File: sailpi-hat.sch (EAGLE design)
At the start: 35 parts, among them X1 PIN20X2, X2 MPT0.5/8-2.54, X3 MPT0.5/8-2.54

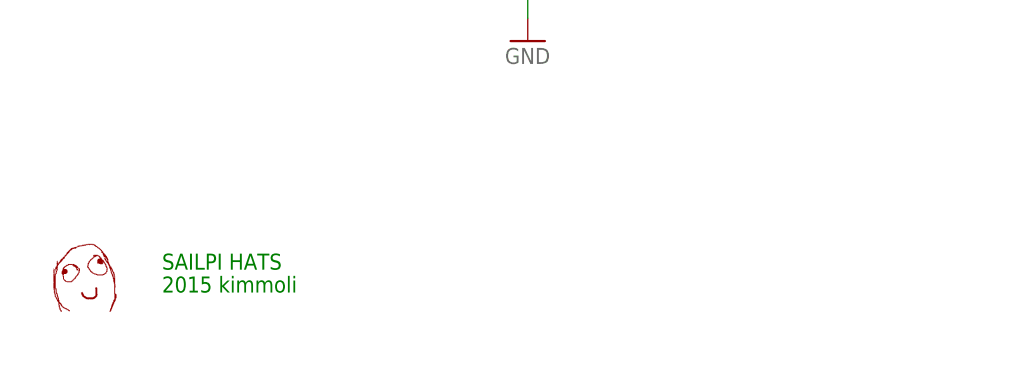
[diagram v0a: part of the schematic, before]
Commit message: add schema and layout pdf, gerbers
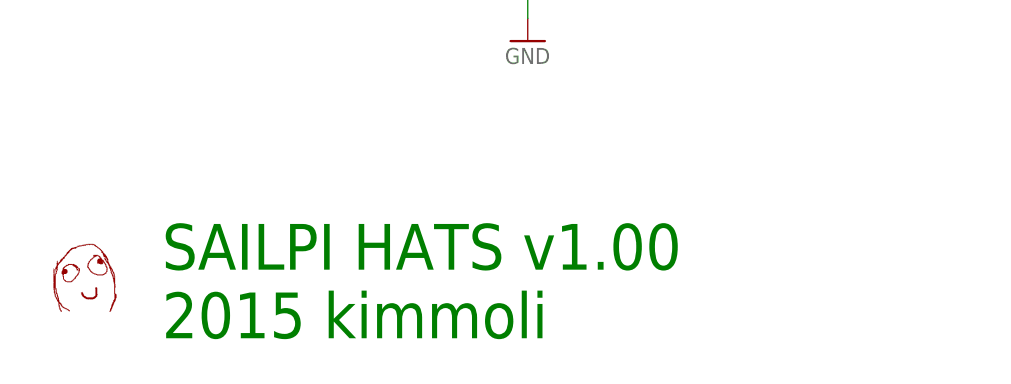
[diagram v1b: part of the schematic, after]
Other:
- note added: "SAILPI HATS v1.00"
- note removed: "SAILPI HATS"
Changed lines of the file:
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@@
 <text x="274.32" y="233.68" size="1.778" layer="91">MCP3021A0T-E/OT</text>
 <text x="274.32" y="238.76" size="1.778" layer="91">i2c address 48</text>
-<text x="58.42" y="15.24" size="1.778" layer="91">SAILPI HATS</text>
-<text x="58.42" y="12.7" size="1.778" layer="91">2015 kimmoli</text>
+<text x="58.42" y="15.24" size="5.08" layer="91">SAILPI HATS v1.00</text>
+<text x="58.42" y="7.62" size="5.08" layer="91">2015 kimmoli</text>
 </plain>
 <instances>
